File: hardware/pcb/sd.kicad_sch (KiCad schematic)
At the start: 17 parts, among them J6 Micro_SD_Card_Det1, J7 Micro_SD_Card_Det1

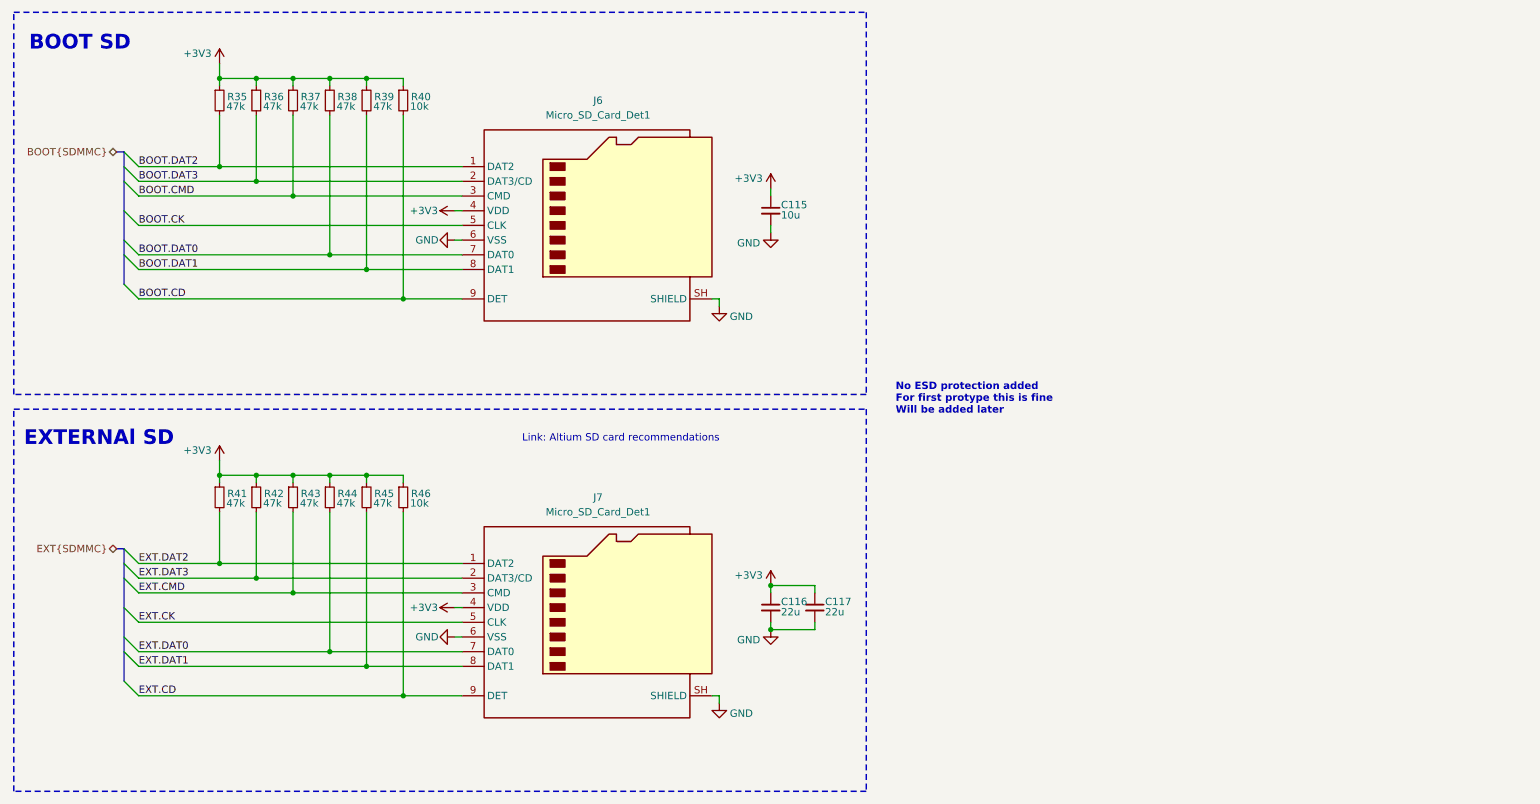
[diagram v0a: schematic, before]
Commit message: added a bunch testpoints
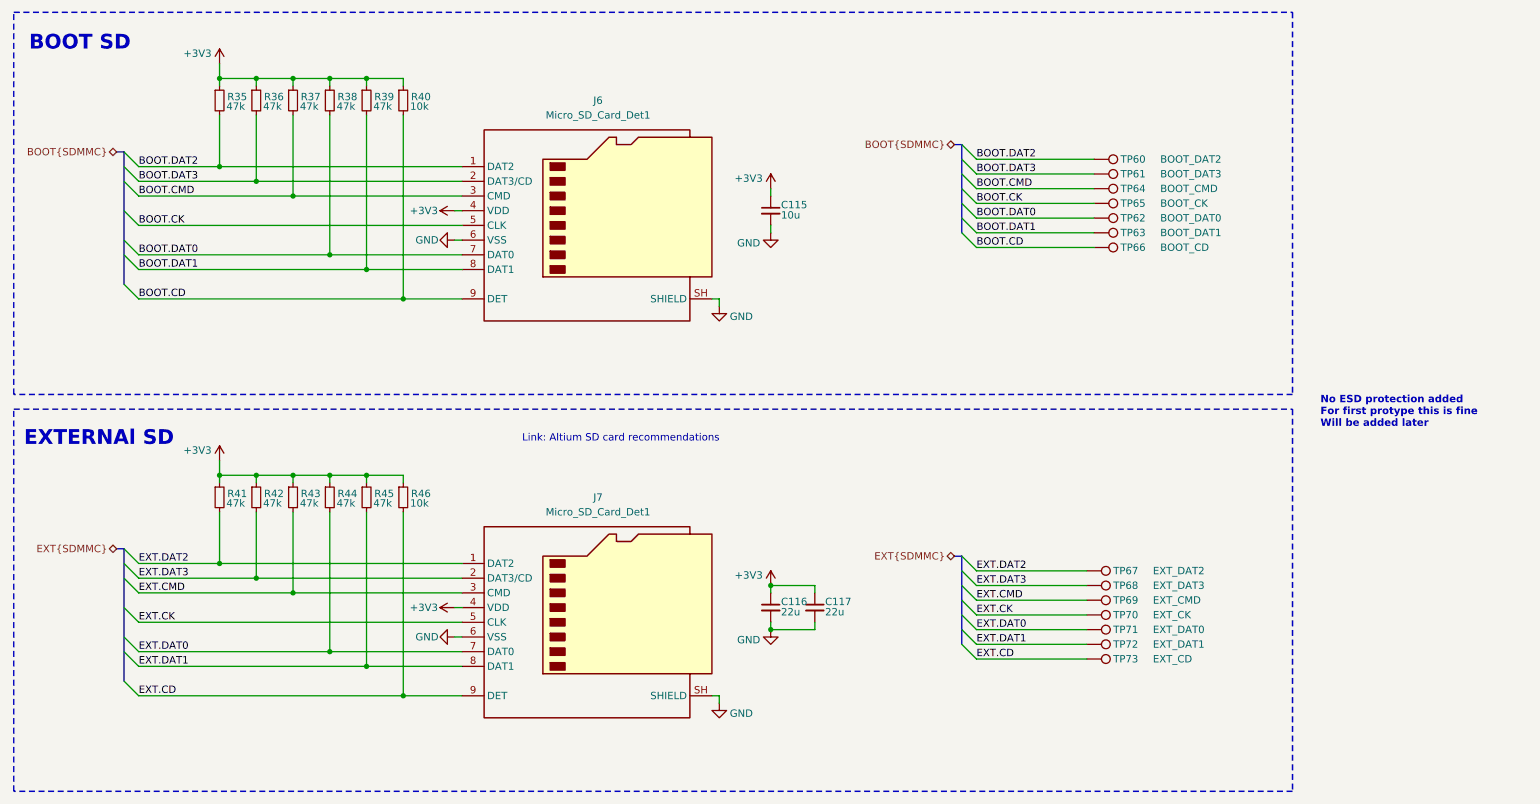
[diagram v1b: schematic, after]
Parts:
- added TP60: BOOT_DAT2, TestPoint:TestPoint_Pad_D1.0mm, symbol Connector:TestPoint
- added TP61: BOOT_DAT3, TestPoint:TestPoint_Pad_D1.0mm, symbol Connector:TestPoint
- added TP62: BOOT_DAT0, TestPoint:TestPoint_Pad_D1.0mm, symbol Connector:TestPoint
- added TP63: BOOT_DAT1, TestPoint:TestPoint_Pad_D1.0mm, symbol Connector:TestPoint
- added TP64: BOOT_CMD, TestPoint:TestPoint_Pad_D1.0mm, symbol Connector:TestPoint
- added TP65: BOOT_CK, TestPoint:TestPoint_Pad_D1.0mm, symbol Connector:TestPoint
- added TP66: BOOT_CD, TestPoint:TestPoint_Pad_D1.0mm, symbol Connector:TestPoint
- added TP67: EXT_DAT2, TestPoint:TestPoint_Pad_D1.0mm, symbol Connector:TestPoint
- added TP68: EXT_DAT3, TestPoint:TestPoint_Pad_D1.0mm, symbol Connector:TestPoint
- added TP69: EXT_CMD, TestPoint:TestPoint_Pad_D1.0mm, symbol Connector:TestPoint
- added TP70: EXT_CK, TestPoint:TestPoint_Pad_D1.0mm, symbol Connector:TestPoint
- added TP71: EXT_DAT0, TestPoint:TestPoint_Pad_D1.0mm, symbol Connector:TestPoint
- added TP72: EXT_DAT1, TestPoint:TestPoint_Pad_D1.0mm, symbol Connector:TestPoint
- added TP73: EXT_CD, TestPoint:TestPoint_Pad_D1.0mm, symbol Connector:TestPoint
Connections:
- net BOOT.CD: now also TP66.1
- net BOOT.CK: now also TP65.1
- net BOOT.CMD: now also TP64.1
- net BOOT.DAT0: now also TP62.1
- net BOOT.DAT1: now also TP63.1
- net BOOT.DAT2: now also TP60.1
- net BOOT.DAT3: now also TP61.1
- net EXT.CD: now also TP73.1
- net EXT.CK: now also TP70.1
- net EXT.CMD: now also TP69.1
- net EXT.DAT0: now also TP71.1
- net EXT.DAT1: now also TP72.1
- net EXT.DAT2: now also TP67.1
- net EXT.DAT3: now also TP68.1
